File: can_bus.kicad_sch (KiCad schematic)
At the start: 1 part, among them U8 MCP2562-E-SN

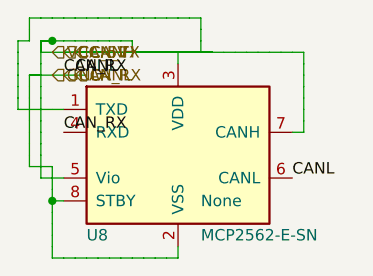
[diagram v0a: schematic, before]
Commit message: рефакторинг проекта и начала прогона тестов
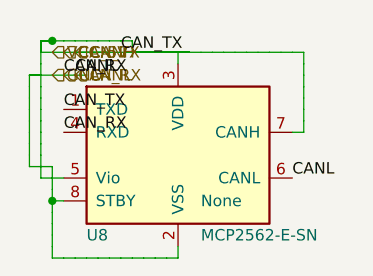
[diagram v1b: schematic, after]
